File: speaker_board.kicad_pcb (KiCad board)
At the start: 2 copper layers, 3 parts, among them J2 MP3_Module

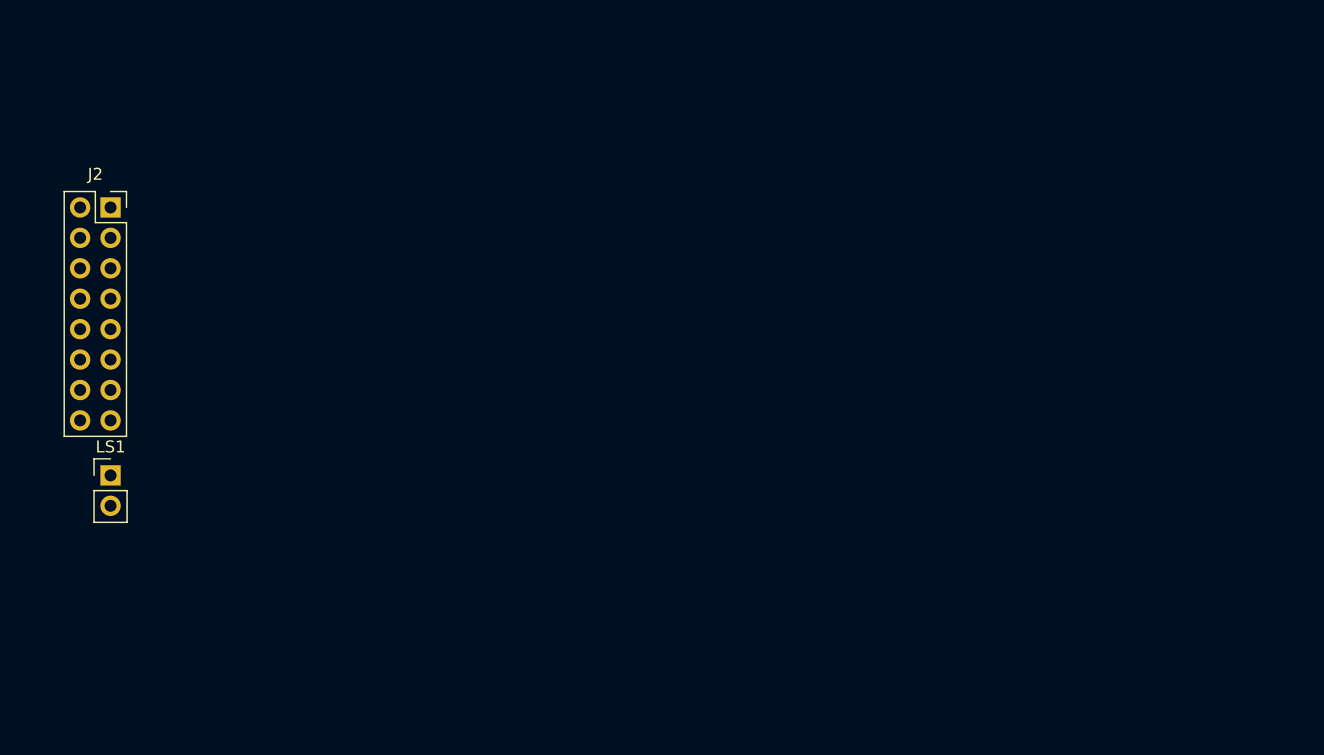
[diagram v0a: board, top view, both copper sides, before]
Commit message: initial pcb
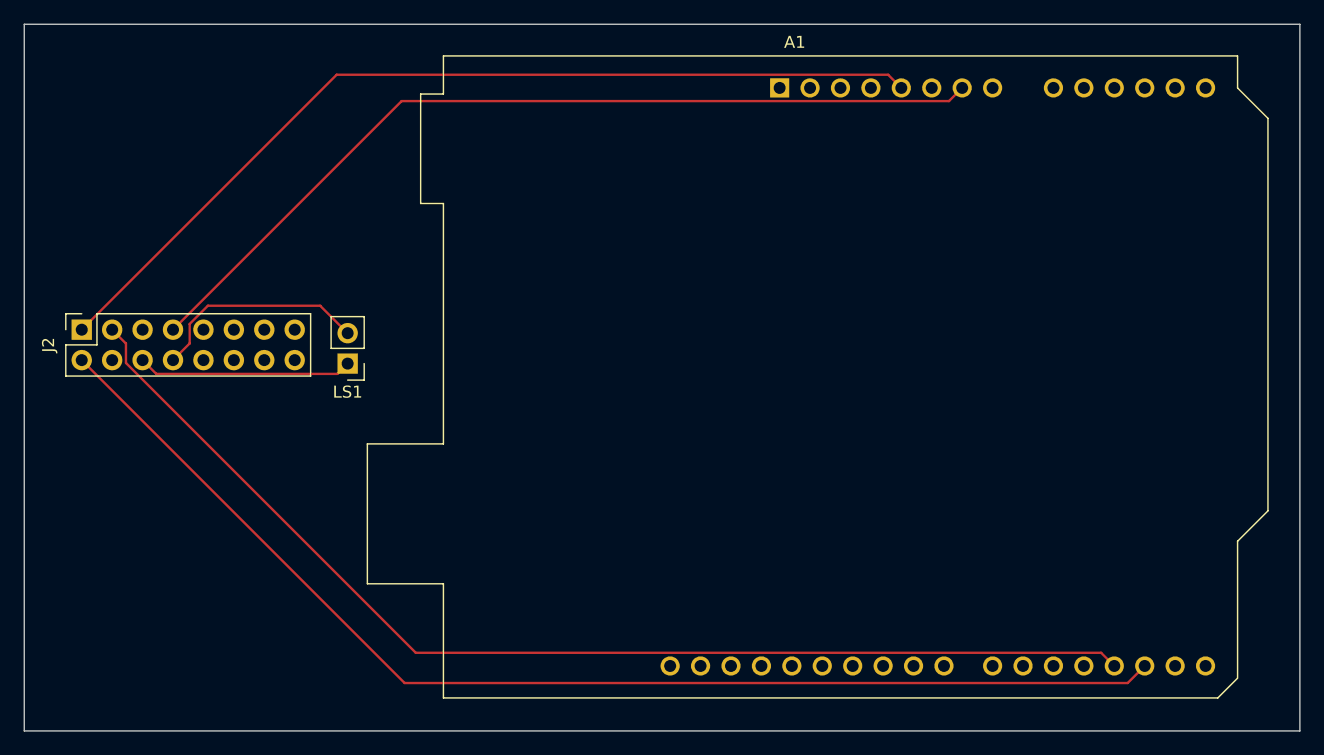
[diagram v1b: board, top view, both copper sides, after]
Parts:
- added A1: Arduino_UNO_R3, Module:Arduino_UNO_R3, F.Cu at (196.6, 57.3)
- moved LS1 21.9 mm to (160.5, 80.3), turned to 180 degrees
- moved J2 10.5 mm to (138.3, 77.5), turned to 90 degrees
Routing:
- net Net-(A1-D2): track 0.00 -> 100.5 mm
- net Net-(A1-D3): track 0.00 -> 96.2 mm
- net +5V: track 0.00 -> 77.7 mm
- net GND: track 0.00 -> 74.2 mm
- net Net-(J2-SPK_2): track 0.00 -> 18.4 mm
- net Net-(J2-SPK_1): track 0.00 -> 18.0 mm
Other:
- board outline added: 106.5 x 59 mm
